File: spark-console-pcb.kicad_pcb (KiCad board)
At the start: 2 copper layers, 105 x 57.5 mm, 33 parts, among them J1 USB_B, J2 PROGRAM, SW1 SW_Push, SW2 SW_Push, SW3 SW_Push, SW4 SW_Push, SW5 SW_Push, SW6 SW_Push, SW7 SW_Push, U1 ATmega328P-P, U2 MAX7221xNG, U3 MAX7221xNG, U4 HL-M1388BRPG, Y1 Crystal

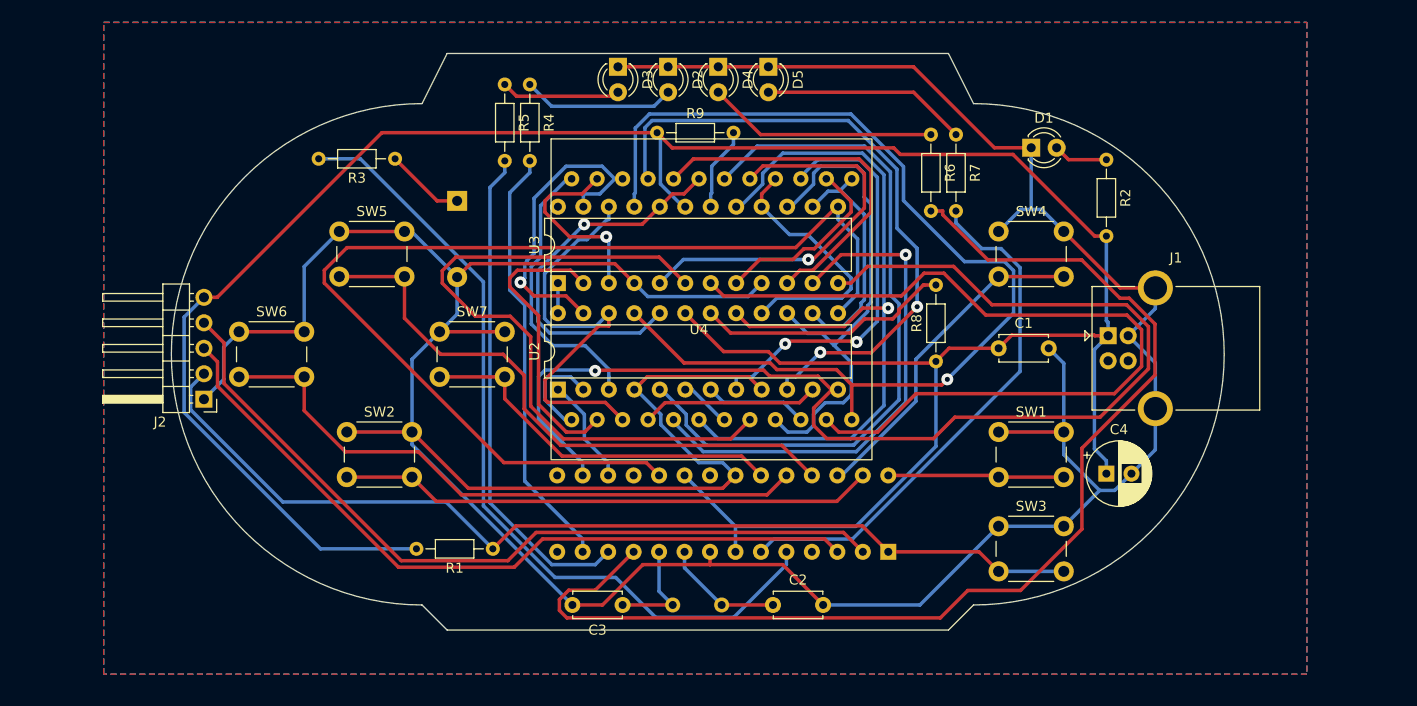
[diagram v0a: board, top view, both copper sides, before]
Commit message: Changes from lazerninja
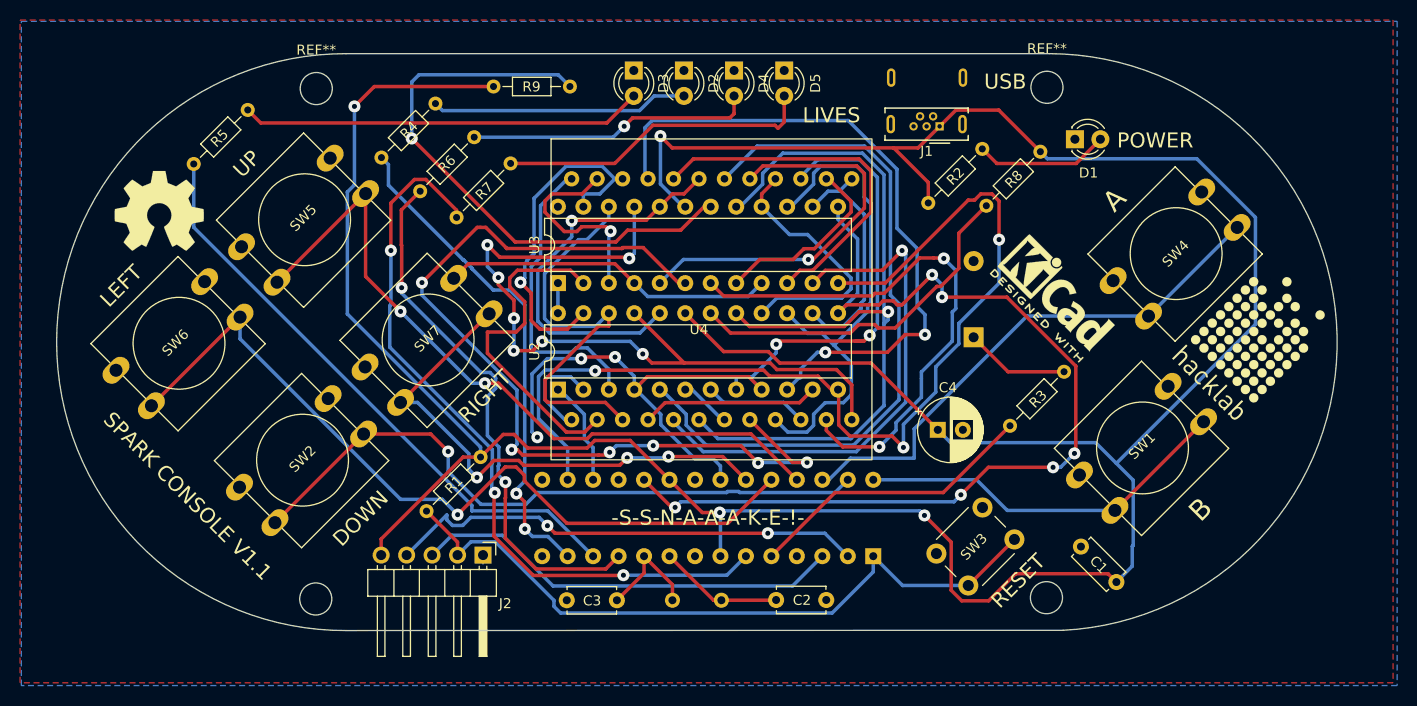
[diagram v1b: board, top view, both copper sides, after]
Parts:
- added ?: , , F.Cu at (184.0, 117.4)
- added ?: , , F.Cu at (175.7, 65.5)
- added ?: , , F.Cu at (168.5, 65.5)
- added ?: , , F.Cu at (111.2, 117.5)
- added G***: LOGO, logo:hacklab_pcb2, F.Cu at (204.6, 91.7)
- added G***: LOGO, logo:hacklab_pcb3, B.Cu at (148.6, 92.5)
- added REF**: MountingHole_3.2mm_M3_ISO7380, MountingHole:MountingHole_3.2mm_M3_ISO7380, F.Cu at (184.1, 66.5)
- added REF**: KiCad-Logo2_5mm_SilkScreen, Symbol:KiCad-Logo2_5mm_SilkScreen, F.Cu at (184.9, 87.4)
- added REF**: MountingHole_3.2mm_M3_ISO7380, MountingHole:MountingHole_3.2mm_M3_ISO7380, F.Cu at (111.2, 66.6)
- added REF**: OSHW-Symbol_8.9x8mm_SilkScreen, Symbol:OSHW-Symbol_8.9x8mm_SilkScreen, F.Cu at (95.5, 78.8)
- J1: footprint Connector_USB:USB_B_OST_USB-B1HSxx_Horizontal -> Connector_USB:USB_Micro-B_Wuerth_614105150721_Vertical
- SW1, SW2, SW4, SW5, SW6, SW7: footprint Button_Switch_THT:SW_PUSH_6mm_H5mm -> Button_Switch_THT:SW_PUSH-12mm
- SW3: footprint Button_Switch_THT:SW_PUSH_6mm_H5mm -> Button_Switch_THT:SW_PUSH_6mm
- moved R3 70.0 mm to (185.8, 94.8), turned to -135 degrees
- moved BZ1 53.3 mm to (176.8, 91.4), turned to 90 degrees
- moved R6 45.5 mm to (127.0, 71.4), turned to -135 degrees
- moved R7 44.5 mm to (130.6, 74.1), turned to -135 degrees
- moved J2 31.9 mm to (127.8, 113.1), turned to -90 degrees
- moved J1 26.8 mm to (173.4, 70.4), turned to 180 degrees
- moved C1 26.1 mm to (191.0, 115.8), turned to 135 degrees
- moved R5 25.8 mm to (104.4, 68.7), turned to -135 degrees
- moved R8 23.4 mm to (183.4, 72.9), turned to -135 degrees
- moved C4 17.4 mm to (173.2, 100.6)
- moved R9 16.9 mm to (128.9, 66.4)
- moved SW6 12.9 mm to (91.2, 94.7), turned to 45 degrees
- moved SW4 12.4 mm to (190.7, 85.8), turned to 45 degrees
- moved R2 12.4 mm to (177.6, 72.6), turned to -135 degrees
- moved SW2 12.0 mm to (103.5, 106.4), turned to 45 degrees
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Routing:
- net GND: track 370.7 -> 82.1 mm, vias 0 -> 3
- net Net-(R6-Pad2): track 117.2 -> 54.1 mm, vias 0 -> 2
- net VCC: track 262.6 -> 324.6 mm, vias 0 -> 4
- net /BUZZER: track 82.1 -> 29.2 mm
- net Net-(R9-Pad2): track 8.32 -> 57.7 mm, vias 0 -> 1
- net Net-(J2-Pad3): track 75.3 -> 43.1 mm
- net Net-(J2-Pad4): track 79.9 -> 48.3 mm, vias 0 -> 2
- net Net-(U3-Pad7): track 85.1 -> 54.9 mm, vias 0 -> 2
- net Net-(D3-Pad2): track 11.9 -> 40.7 mm
- net /RESET: track 99.8 -> 71.4 mm
- net Net-(U2-Pad21): track 106.1 -> 78.1 mm, vias 1 -> 7
- net Net-(R7-Pad2): track 53.1 -> 74.7 mm, vias 0 -> 3
- net Net-(U3-Pad6): track 69.1 -> 90.0 mm, vias 0 -> 6
- net /BTN_LEFT: track 17.6 -> 37.9 mm
- net /BTN_UP: track 33.2 -> 53.5 mm
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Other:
- board size 105 x 57.5 mm -> 127.7 x 57.5 mm
- board text added: "-S-S-N-A-A-A-K-E-!-"
- board text added: "A"
- board text added: "B"
- board text added: "DOWN"
- board text added: "LEFT"
- board text added: "LIVES"
- board text added: "POWER"
- board text added: "RESET"
- board text added: "RIGHT"
- board text added: "SPARK CONSOLE V1.1"
- board text added: "UP"
- board text added: "USB"
